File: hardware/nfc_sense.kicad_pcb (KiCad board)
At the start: 4 copper layers, 18.6 x 43.1 mm, 24 parts, among them U1 TMP117AIDRVR, U2 RF430CL330HIRGTR‎, U3 ATtiny1626-MFR

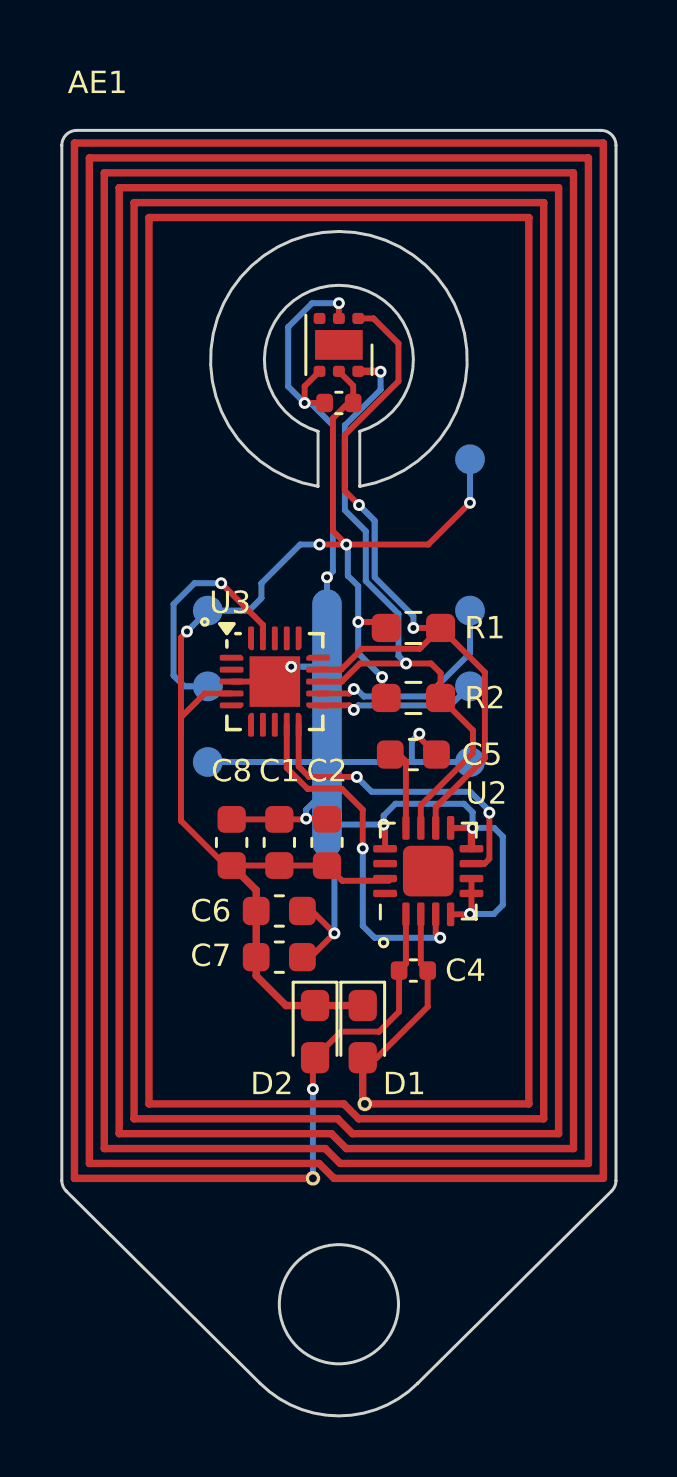
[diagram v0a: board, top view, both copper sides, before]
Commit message: desc + new TP
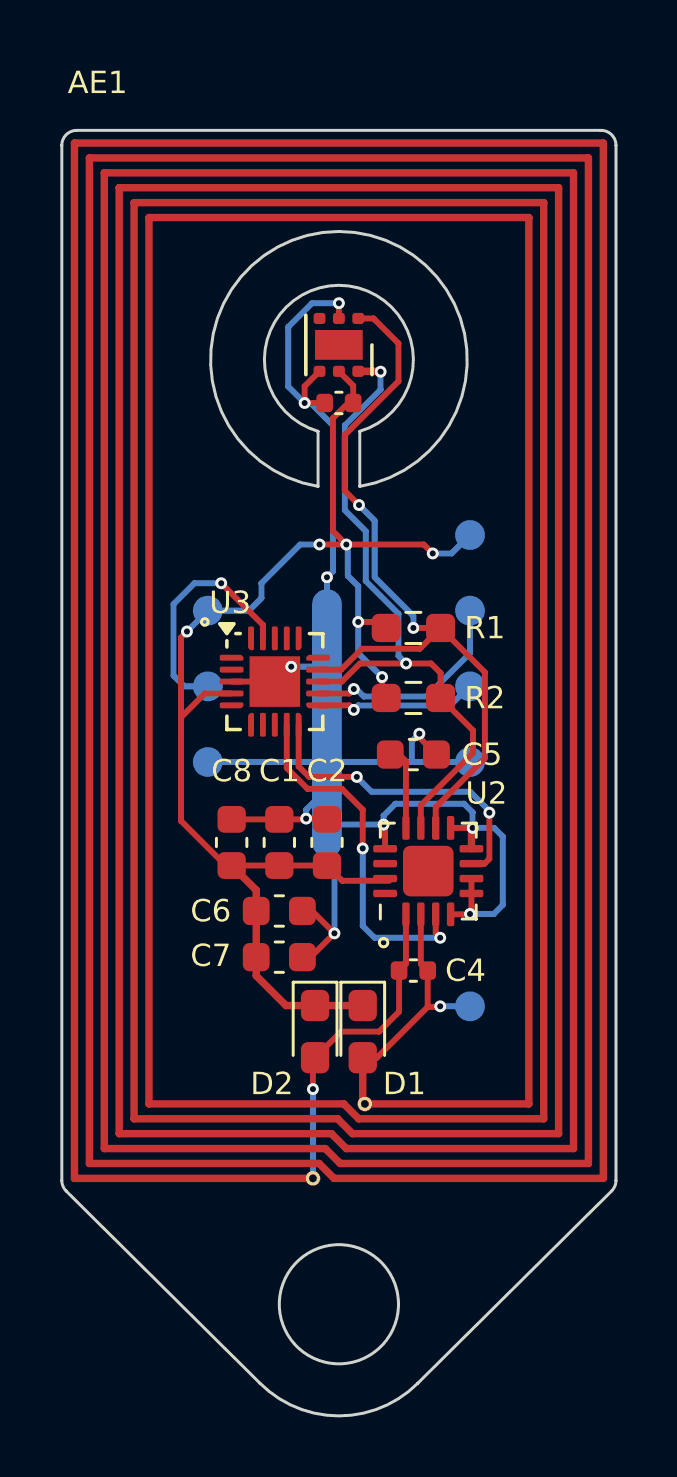
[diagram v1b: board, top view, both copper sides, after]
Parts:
- added TP5: TestPoint, TestPoint:TestPoint_Pad_D1.0mm, B.Cu at (133.9, 60.9)
- U1: footprint unsurv_offline_pcb_footprints:TMP117 WSON-6-1EP_2x2mm_P0.65mm -> unsurv_offline_pcb_footprints:TMP117 WSON-6-1EP_2x2mm_P0.65mm_no_pad_paste
- moved TP4 2.54 mm to (133.9, 45.1)
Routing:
- net VCC: track 51.8 -> 50.2 mm
- net ANT2: track 7.67 -> 9.10 mm, vias 0 -> 1
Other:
- board text added: "VCC TX RX GND NFC"
- board text added: "v 1.0 Made in Germany 11/24"
- board text removed: "VCC TX RX GND"
- board text removed: "v 0.9 pre-production 09/24"
